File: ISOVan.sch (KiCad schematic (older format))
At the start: 14 parts

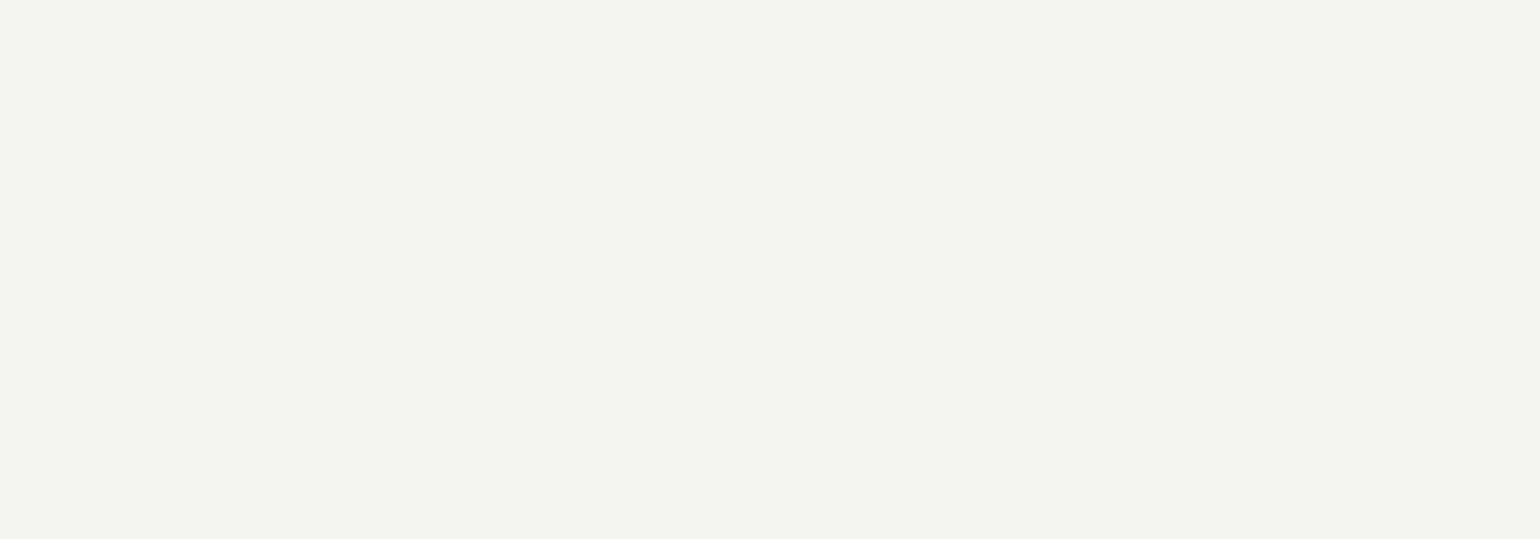
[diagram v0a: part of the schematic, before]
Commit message: start matrix
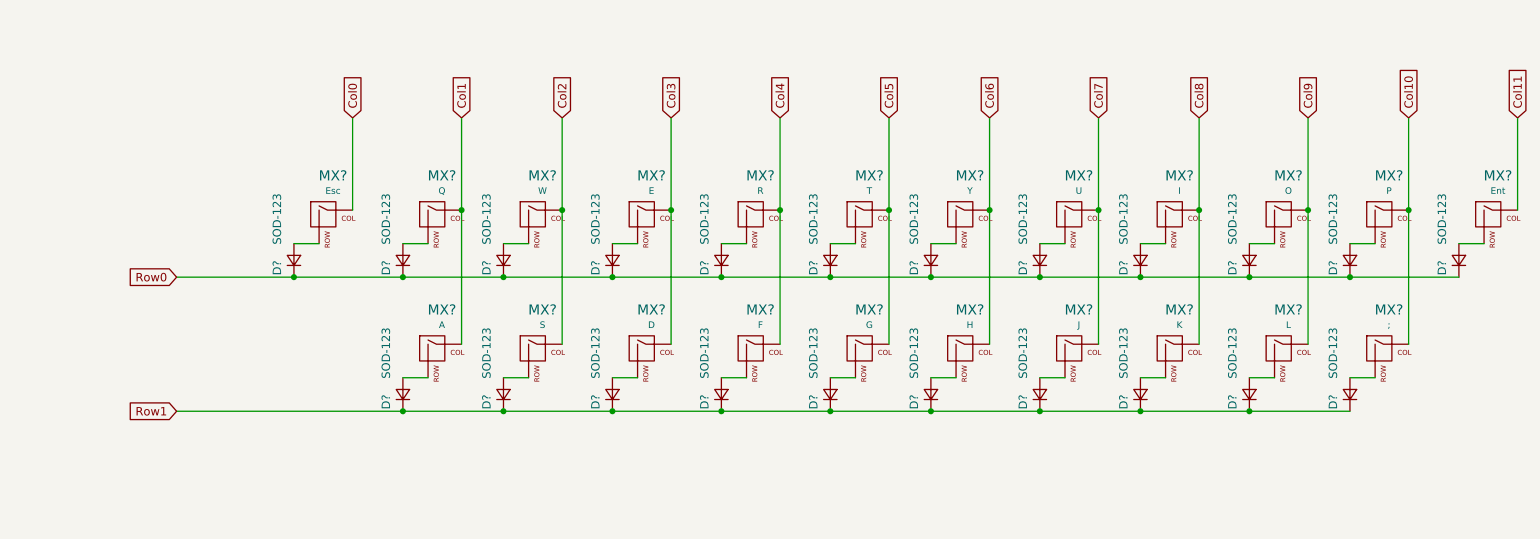
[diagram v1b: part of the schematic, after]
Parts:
- added D? (x22): SOD-123, symbol Device:D_Small
- added MX?: Esc, symbol MX_Alps_Hybrid:MX-NoLED
- added MX?: Q, symbol MX_Alps_Hybrid:MX-NoLED
- added MX?: W, symbol MX_Alps_Hybrid:MX-NoLED
- added MX?: E, symbol MX_Alps_Hybrid:MX-NoLED
- added MX?: R, symbol MX_Alps_Hybrid:MX-NoLED
- added MX?: T, symbol MX_Alps_Hybrid:MX-NoLED
- added MX?: Y, symbol MX_Alps_Hybrid:MX-NoLED
- added MX?: U, symbol MX_Alps_Hybrid:MX-NoLED
- added MX?: I, symbol MX_Alps_Hybrid:MX-NoLED
- added MX?: O, symbol MX_Alps_Hybrid:MX-NoLED
- added MX?: P, symbol MX_Alps_Hybrid:MX-NoLED
- added MX?: Ent, symbol MX_Alps_Hybrid:MX-NoLED
- added MX?: ;, symbol MX_Alps_Hybrid:MX-NoLED
- added MX?: L, symbol MX_Alps_Hybrid:MX-NoLED
- added MX?: K, symbol MX_Alps_Hybrid:MX-NoLED
- added MX?: J, symbol MX_Alps_Hybrid:MX-NoLED
- added MX?: H, symbol MX_Alps_Hybrid:MX-NoLED
- added MX?: G, symbol MX_Alps_Hybrid:MX-NoLED
- added MX?: F, symbol MX_Alps_Hybrid:MX-NoLED
- added MX?: D, symbol MX_Alps_Hybrid:MX-NoLED
- added MX?: S, symbol MX_Alps_Hybrid:MX-NoLED
- added MX?: A, symbol MX_Alps_Hybrid:MX-NoLED
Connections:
- new net: D?.2 (A), MX?.2 (ROW) (x22)
- new net Col0: MX?.1 (COL)
- new net Col1: MX?.1 (COL), MX?.1 (COL)
- new net Col10: MX?.1 (COL), MX?.1 (COL)
- new net Col11: MX?.1 (COL)
- new net Col2: MX?.1 (COL), MX?.1 (COL)
- new net Col3: MX?.1 (COL), MX?.1 (COL)
- new net Col4: MX?.1 (COL), MX?.1 (COL)
- new net Col5: MX?.1 (COL), MX?.1 (COL)
- new net Col6: MX?.1 (COL), MX?.1 (COL)
- new net Col7: MX?.1 (COL), MX?.1 (COL)
- new net Col8: MX?.1 (COL), MX?.1 (COL)
- new net Col9: MX?.1 (COL), MX?.1 (COL)
- new net Row0: D?.1 (K), D?.1 (K), D?.1 (K), D?.1 (K), D?.1 (K), D?.1 (K), D?.1 (K), D?.1 (K), D?.1 (K), D?.1 (K), D?.1 (K), D?.1 (K)
- new net Row1: D?.1 (K), D?.1 (K), D?.1 (K), D?.1 (K), D?.1 (K), D?.1 (K), D?.1 (K), D?.1 (K), D?.1 (K), D?.1 (K)

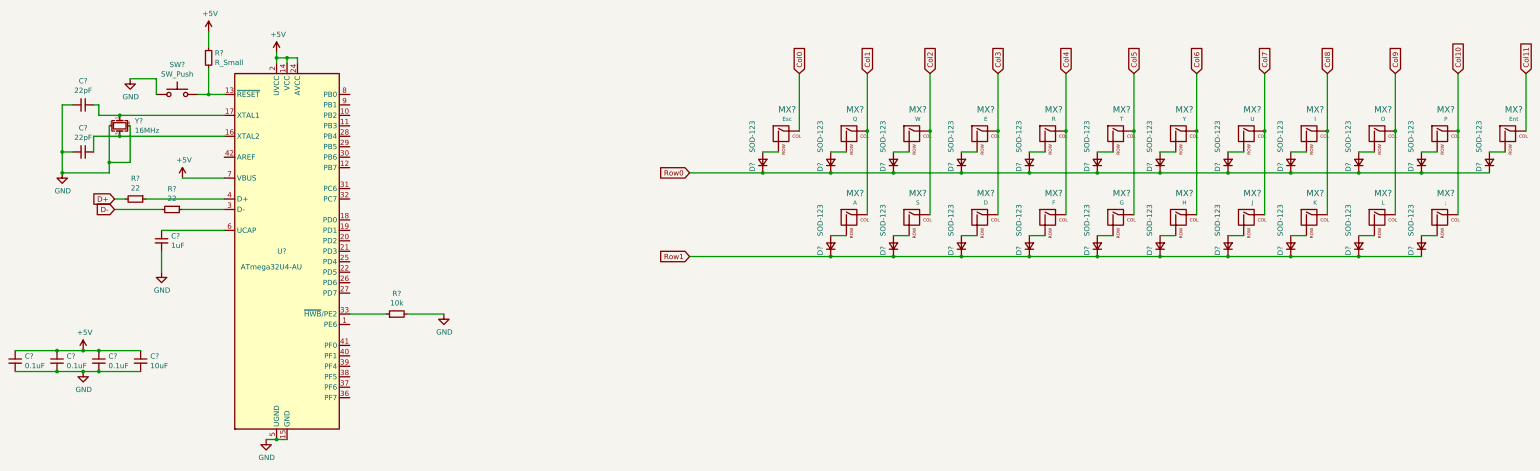
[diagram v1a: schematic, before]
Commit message: Finish matrix
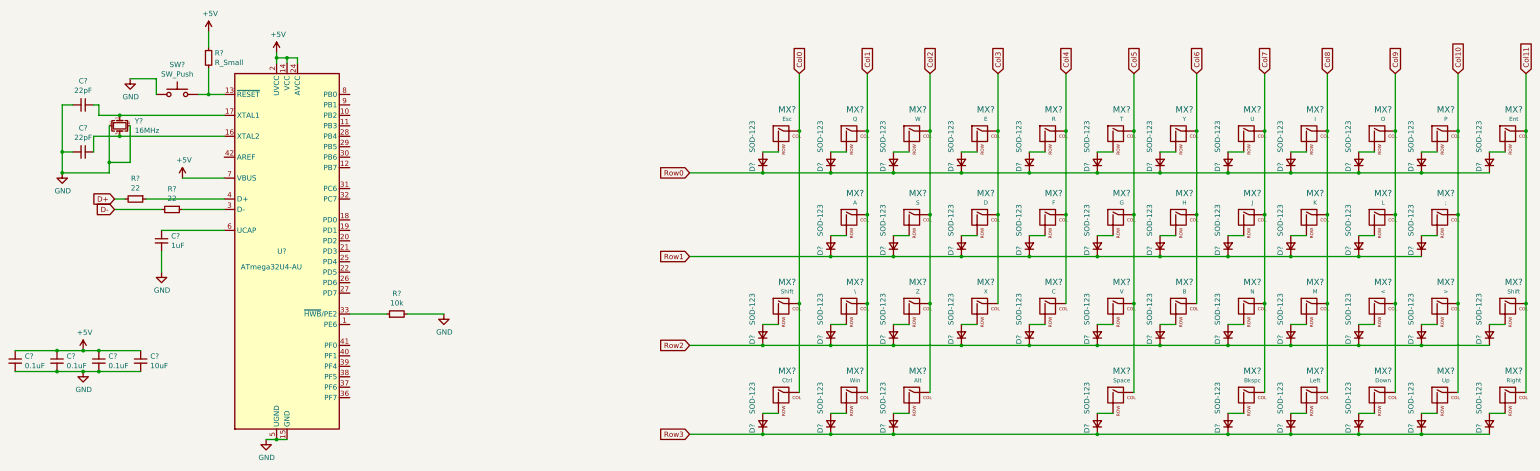
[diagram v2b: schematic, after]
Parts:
- added D? (x21): SOD-123, symbol Device:D_Small
- added MX? (x2): Shift, symbol MX_Alps_Hybrid:MX-NoLED
- added MX?: >, symbol MX_Alps_Hybrid:MX-NoLED
- added MX?: <, symbol MX_Alps_Hybrid:MX-NoLED
- added MX?: M, symbol MX_Alps_Hybrid:MX-NoLED
- added MX?: N, symbol MX_Alps_Hybrid:MX-NoLED
- added MX?: B, symbol MX_Alps_Hybrid:MX-NoLED
- added MX?: V, symbol MX_Alps_Hybrid:MX-NoLED
- added MX?: C, symbol MX_Alps_Hybrid:MX-NoLED
- added MX?: X, symbol MX_Alps_Hybrid:MX-NoLED
- added MX?: Z, symbol MX_Alps_Hybrid:MX-NoLED
- added MX?: \\, symbol MX_Alps_Hybrid:MX-NoLED
- added MX?: Ctrl, symbol MX_Alps_Hybrid:MX-NoLED
- added MX?: Win, symbol MX_Alps_Hybrid:MX-NoLED
- added MX?: Alt, symbol MX_Alps_Hybrid:MX-NoLED
- added MX?: Space, symbol MX_Alps_Hybrid:MX-NoLED
- added MX?: Bkspc, symbol MX_Alps_Hybrid:MX-NoLED
- added MX?: Left, symbol MX_Alps_Hybrid:MX-NoLED
- added MX?: Down, symbol MX_Alps_Hybrid:MX-NoLED
- added MX?: Up, symbol MX_Alps_Hybrid:MX-NoLED
- added MX?: Right, symbol MX_Alps_Hybrid:MX-NoLED
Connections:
- net Col0: now also MX?.1 (COL), MX?.1 (COL)
- net Col1: now also MX?.1 (COL), MX?.1 (COL)
- net Col10: now also MX?.1 (COL), MX?.1 (COL)
- net Col11: now also MX?.1 (COL), MX?.1 (COL)
- net Col2: now also MX?.1 (COL), MX?.1 (COL)
- net Col3: now also MX?.1 (COL)
- net Col4: now also MX?.1 (COL)
- net Col5: now also MX?.1 (COL), MX?.1 (COL)
- net Col6: now also MX?.1 (COL)
- net Col7: now also MX?.1 (COL), MX?.1 (COL)
- net Col8: now also MX?.1 (COL), MX?.1 (COL)
- net Col9: now also MX?.1 (COL), MX?.1 (COL)
- new net: D?.2 (A), MX?.2 (ROW) (x21)
- new net Row2: D?.1 (K), D?.1 (K), D?.1 (K), D?.1 (K), D?.1 (K), D?.1 (K), D?.1 (K), D?.1 (K), D?.1 (K), D?.1 (K), D?.1 (K), D?.1 (K)
- new net Row3: D?.1 (K), D?.1 (K), D?.1 (K), D?.1 (K), D?.1 (K), D?.1 (K), D?.1 (K), D?.1 (K), D?.1 (K)
